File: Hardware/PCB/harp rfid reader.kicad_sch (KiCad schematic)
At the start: 22 parts, among them IC1 FT232RL, IC2 LP5907MFX-3.3, J1 USB4105-GF-A

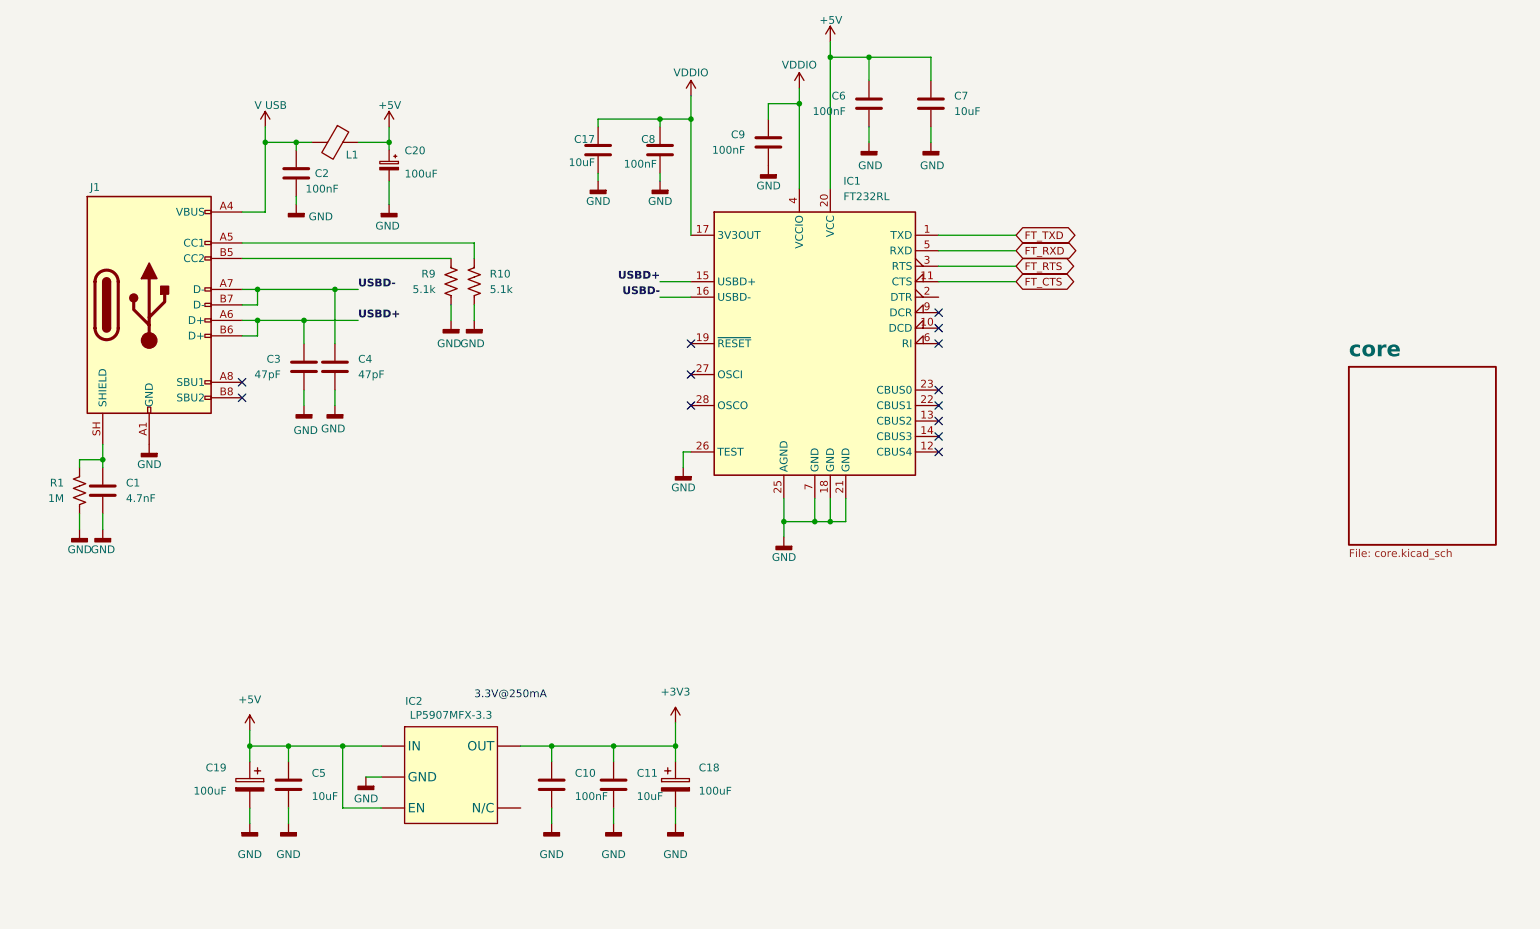
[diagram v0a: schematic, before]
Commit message: versão 1.3 final & ficheiros de manufacturing
- ainda sem revisão do Filipe
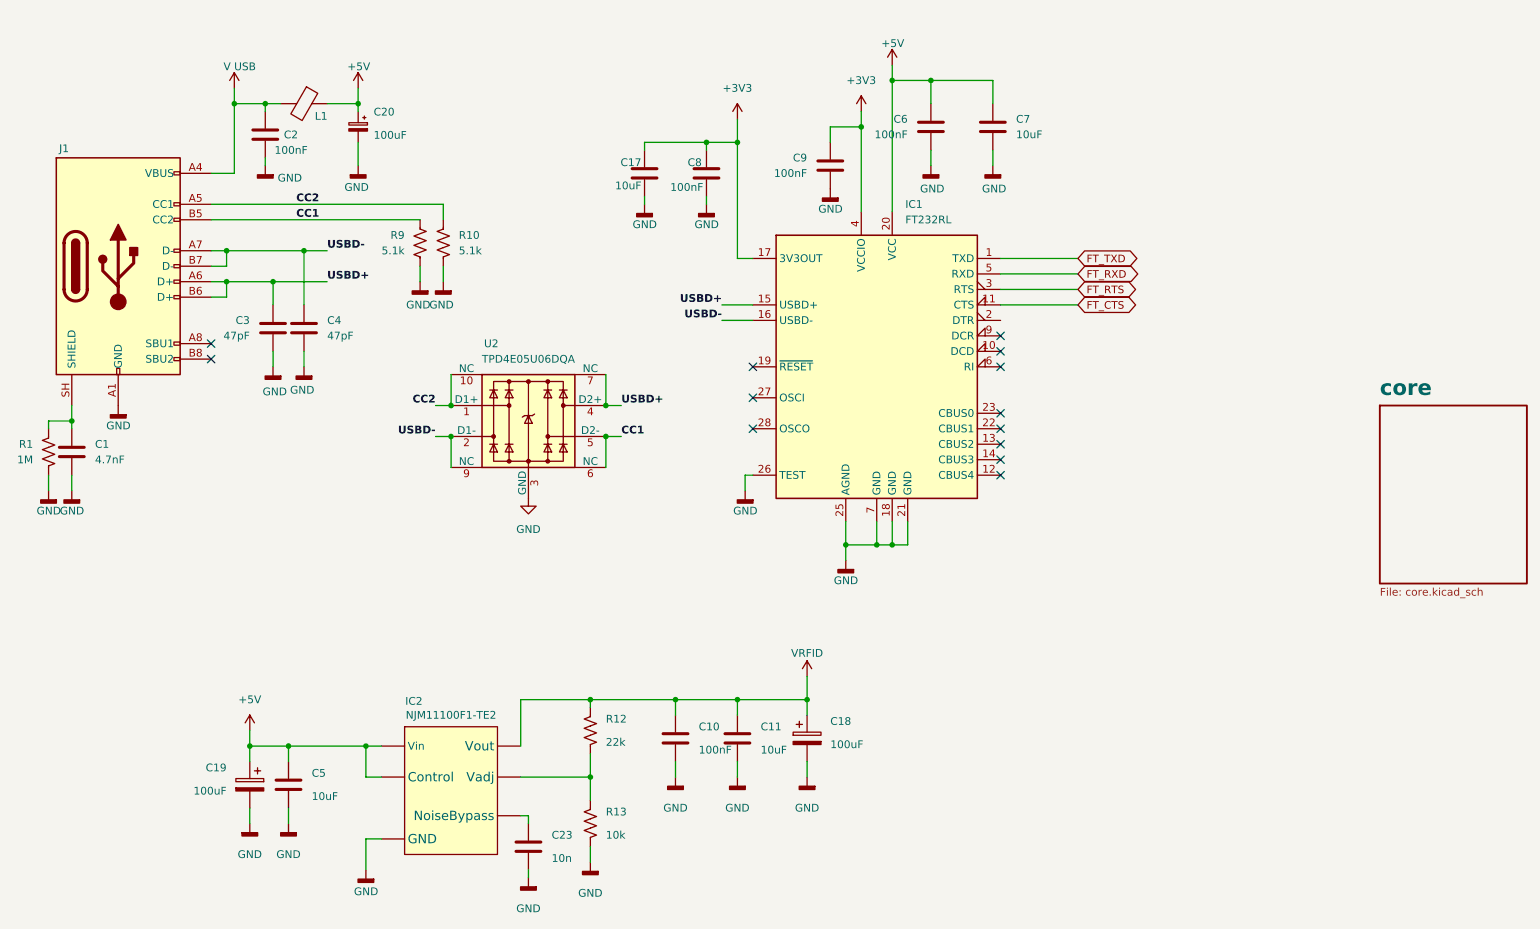
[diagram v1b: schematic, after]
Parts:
- added C23: 10n, Capacitor_SMD:C_0402_1005Metric, symbol Device:C
- added R12: 22k, Resistor_SMD:R_0402_1005Metric, symbol Device:R_US
- added R13: 10k, Resistor_SMD:R_0402_1005Metric, symbol Device:R_US
- added U2: TPD4E05U06DQA, Package_SON:USON-10_2.5x1.0mm_P0.5mm, symbol Power_Protection:TPD4E05U06DQA
- C1: OEPSPN (none) -> OEPS010017; TempCo (none) -> X7R; Tolerance (none) -> ±10%; Voltage (none) -> 100V
- C10, C2, C6, C8, C9: OEPSPN (none) -> OEPS010016; TempCo (none) -> X7R; Tolerance (none) -> ±10%; Voltage (none) -> 50V
- C11, C17, C5, C7: OEPSPN (none) -> OEPS010015; TempCo (none) -> X5R; Tolerance (none) -> ±20%; Voltage (none) -> 16V
- C18, C19, C20: OEPSPN (none) -> OEPS210002; TempCo (none) -> TANT A; Tolerance (none) -> ±20%; Voltage (none) -> 10V
- C3, C4: OEPSPN (none) -> OEPS010011; TempCo (none) -> C0G; Tolerance (none) -> ±5%; Voltage (none) -> 50V
- IC1: MPN FT232RL-REEL ?? -> FT232RL-REEL; OEPSPN (none) -> OEPS080013
- IC2: value LP5907MFX-3.3 -> NJM11100F1-TE2; footprint Package_TO_SOT_SMD:TSOT-23-5 -> Package_TO_SOT_SMD:SOT-23-6; symbol harp rfid reader:TLV700XX -> harp rfid reader:NJM11100; MPN (none) -> NJM11100F1-TE2; OEPSPN (none) -> OEPS080147
- L1: value 40R@100MHz -> MI0805K400R-10; OEPSPN (none) -> OEPS040003
- R1: OEPSPN (none) -> OEPS020026; Tolerance (none) -> ±1%
- R10, R9: Tolerance (none) -> ±1%
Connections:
- net VDDIO is gone; now on net +3V3: C17.1, C8.1, C9.1, IC1.17 (3V3OUT), IC1.4 (VCCIO)
- net +3V3: no longer C10.1, C11.1, C18.1, IC2.5 (OUT)
- net +5V: now also IC2.6 (Vin); no longer IC2.3 (EN)
- net GND: now also C23.2, R13.2, U2.3 (GND), U2.8 (GND)
- net USBD+: now also U2.4 (D2+), U2.7 (NC)
- net USBD-: now also U2.2 (D1-), U2.9 (NC)
- net CC2: now reaches J1.A5 (CC1), R10.1
- net CC2: now also U2.1 (D1+), U2.10 (NC)
- net CC1: now reaches J1.B5 (CC2), R9.1
- net CC1: now also U2.5 (D2-), U2.6 (NC)
- net VRFID: now reaches IC2.4 (Vout)
- net VRFID: now also C10.1, C11.1, C18.1, R12.1
- new net: IC2.5 (Vadj), R12.2, R13.1
- new net: C23.1, IC2.3 (NoiseBypass)
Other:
- note removed: "3.3V@250mA"
- moved on the sheet: C1, C10, C11, C17, C18, C2, C20, C3, C4, C6, C7, C8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
